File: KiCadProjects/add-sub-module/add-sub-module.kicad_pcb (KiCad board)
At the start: 2 copper layers, 56 x 68 mm, 32 parts, among them J1 2x4_Header, J2 1x2_Header, M1 MountingHole_2.2mm_M2_Pad, M2 MountingHole_2.2mm_M2_Pad, M3 MountingHole_2.2mm_M2_Pad, M4 MountingHole_2.2mm_M2_Pad

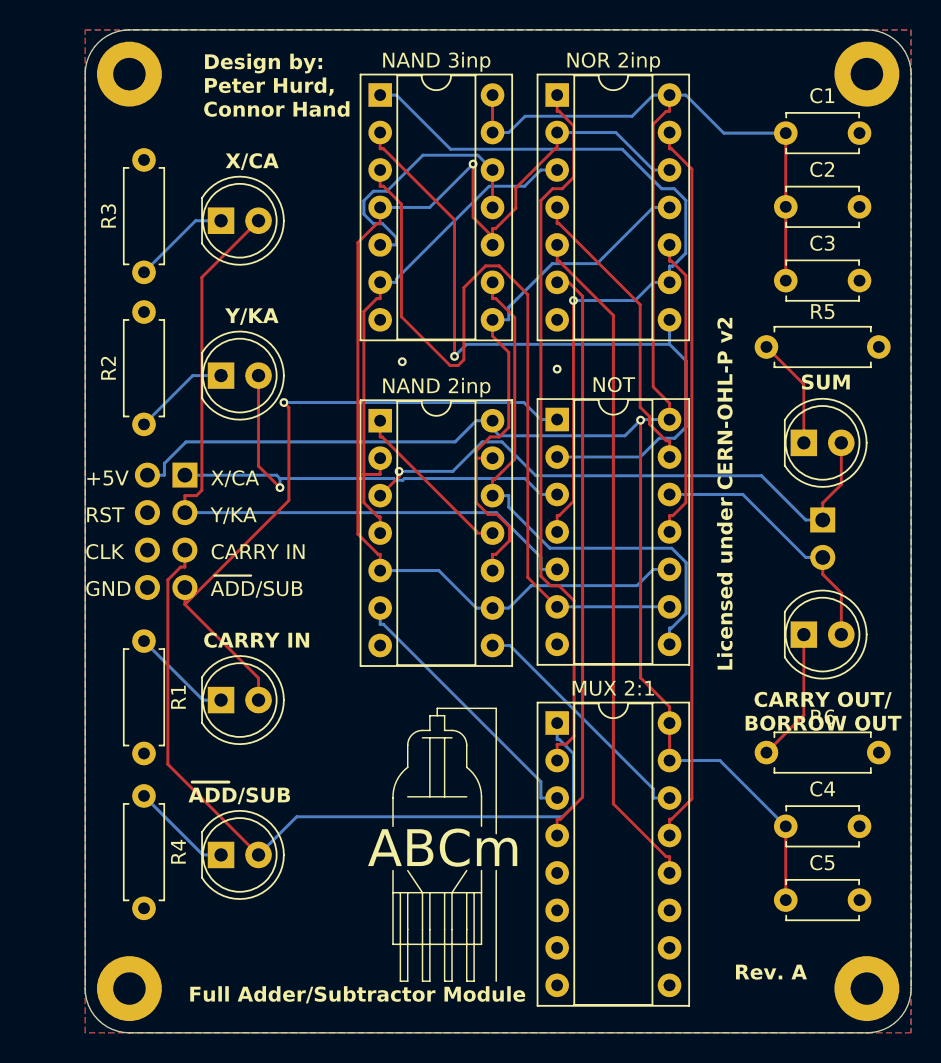
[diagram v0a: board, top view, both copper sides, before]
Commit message: final updates for Revision A
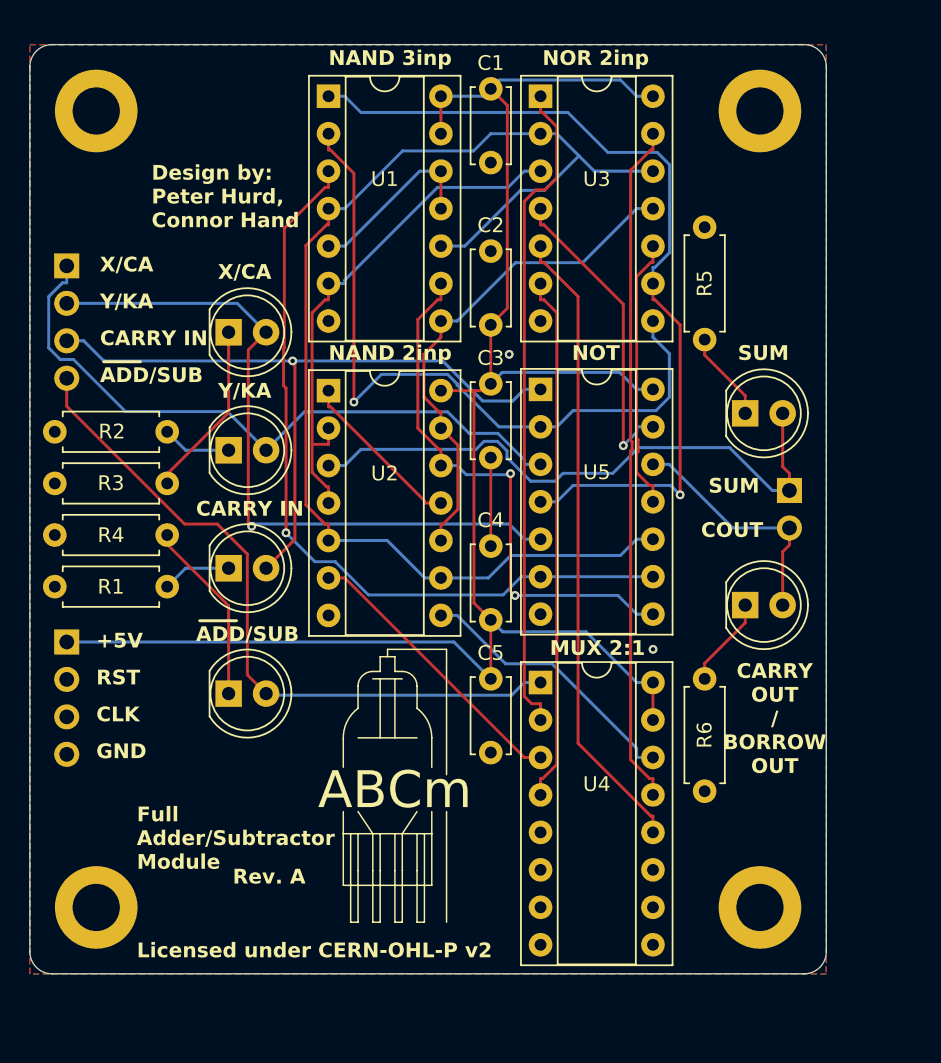
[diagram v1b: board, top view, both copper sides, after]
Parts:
- removed M1, M2, M3, M4: MountingHole_2.2mm_M2_Pad, MountingHole:MountingHole_2.2mm_M2_Pad
- added H1: MountingHole_Pad, MountingHole:MountingHole_3.2mm_M3_DIN965_Pad, F.Cu at (100.2, 67.0)
- added H2: MountingHole_Pad, MountingHole:MountingHole_3.2mm_M3_DIN965_Pad, F.Cu at (145.2, 67.0)
- added H3: MountingHole_Pad, MountingHole:MountingHole_3.2mm_M3_DIN965_Pad, F.Cu at (100.2, 121.0)
- added H4: MountingHole_Pad, MountingHole:MountingHole_3.2mm_M3_DIN965_Pad, F.Cu at (145.2, 121.0)
- added J3: Conn_01x02_Pin, Connector_PinHeader_2.54mm:PinHeader_1x02_P2.54mm_Vertical, B.Cu at (147.2, 92.7)
- C1, C2, C3, C4, C5: footprint Capacitor_THT:C_Disc_D4.7mm_W2.5mm_P5.00mm -> Capacitor_THT:C_Disc_D5.0mm_W2.5mm_P5.00mm
- J1: value 2x4_Header -> Conn_01x04_Pin; footprint Connector_PinHeader_2.54mm:PinHeader_2x04_P2.54mm_Vertical -> Connector_PinHeader_2.54mm:PinHeader_1x04_P2.54mm_Vertical
- J2: value 1x2_Header -> Conn_01x04_Pin; footprint Connector_PinHeader_2.54mm:PinHeader_1x02_P2.54mm_Vertical -> Connector_PinHeader_2.54mm:PinHeader_1x04_P2.54mm_Vertical
- R1, R2, R3, R4, R5, R6: value 1k -> 330
- U1: renamed from NAND 3inp
- U2: renamed from NAND 2inp
- U3: renamed from NOR 2inp
- U4: renamed from MUX 2:1
- moved J2 54.1 mm to (98.2, 77.5)
- moved G*** 30.6 mm to (146.0, 76.0)
- moved C5 25.0 mm to (127.0, 105.5), turned to -90 degrees
- moved C4 24.4 mm to (127.0, 101.5), turned to 90 degrees
- moved C2 21.5 mm to (127.0, 81.5), turned to 90 degrees
- moved C3 21.2 mm to (127.0, 85.5), turned to -90 degrees
- moved C1 20.2 mm to (127.0, 65.5), turned to -90 degrees
- moved R4 17.8 mm to (105.1, 95.8), turned to 180 degrees
- moved R3 14.4 mm to (105.1, 92.2), turned to 180 degrees
- moved J1 13.9 mm to (98.2, 103.0)
- moved D4 11.0 mm to (109.2, 106.5)
- moved D1 8.95 mm to (109.2, 98.0)
- moved REF** 7.60 mm to (108.5, 74.2)
- moved D3 7.58 mm to (109.2, 82.0)
- moved R6 6.52 mm to (141.5, 105.5), turned to -90 degrees
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- renumbered NOT to U5
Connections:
- J1 pad 1: KA -> +5V
- J1 pad 2: +5V -> CLK
- J1 pad 3: CA -> RST
- J1 pad 4: RST -> GND
- J2 pad 1: SUM -> KA
- J2 pad 2: COUT -> CA
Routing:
- net +5V: track 135.0 -> 119.2 mm, vias 1 -> 0
- net KA: track 34.7 -> 45.2 mm, vias 1 -> 0
- net Net-(U1-1Y): track 18.3 -> 12.3 mm
- net Net-(U1-2B): track 79.1 -> 85.2 mm, vias 1 -> 0
- net GND: track 0.00 -> 6.00 mm
- net Net-(U1-1A): track 53.1 -> 59.0 mm
- net Net-(D4-K): track 6.88 -> 12.5 mm
- net ADD/SUB: track 52.7 -> 47.3 mm
- net Net-(D3-K): track 6.67 -> 12.0 mm
- net Net-(U3-1Y): track 49.1 -> 44.9 mm
- net Net-(U3-2B): track 39.5 -> 35.8 mm
- net CARRY: track 45.5 -> 49.1 mm
- net Net-(U1-2A): track 56.7 -> 53.1 mm, vias 0 -> 1
- net Net-(D6-K): track 9.05 -> 6.14 mm
- net Net-(U1-3Y): track 37.4 -> 34.5 mm
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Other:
- board size 56 x 68 mm -> 54 x 63 mm
- board text added: "CARRY OUT / BORROW OUT"
- board text added: "COUT"
- board text added: "MUX 2:1"
- board text added: "NAND 2inp"
- board text added: "NAND 3inp"
- board text added: "NOR 2inp"
- board text added: "NOT"
- board text removed: "CARRY OUT/ BORROW OUT"

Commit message: FINAL FINAL final updates for Rev. A
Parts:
- U1: value CD74HCT10E -> IC-14P
- U2: value SN74HCT00N -> IC-14P
- U3: value SN74HCT02N -> IC-14P
- U4: value SN74HCT257N -> IC-16P
- U5: value CD74HCT04E -> IC-14P
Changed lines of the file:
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@@
 			)
 		)
-		(property "Value" "SN74HCT257N"
+		(property "Value" "IC-16P"
 			(at 3.81 20.11 0)
 			(layer "F.Fab")
@@
 			)
 		)
-		(property "Datasheet" "SN74HCT257N"
+		(property "Datasheet" ""
 			(at 0 0 0)
 			(unlocked yes)
@@
 			)
 		)
-		(property "Description" ""
+		(property "Description" "SN74HCT257N"
 			(at 0 0 0)
 			(unlocked yes)
@@
 			)
 		)
-		(property "Value" "CD74HCT10E"
+		(property "Value" "IC-14P"
 			(at 3.81 17.57 0)
 			(layer "F.Fab")
@@
 			)
 		)
-		(property "Datasheet" "CD74HCT10E"
+		(property "Datasheet" ""
 			(at 0 0 0)
 			(unlocked yes)
@@
 			)
 		)
-		(property "Description" ""
+		(property "Description" "CD74HCT10E"
 			(at 0 0 0)
 			(unlocked yes)
@@
 			)
 		)
-		(property "Value" "SN74HCT00N"
+		(property "Value" "IC-14P"
 			(at 3.81 17.57 0)
 			(layer "F.Fab")
@@
 			)
 		)
-		(property "Datasheet" "SN74HCT00N"
+		(property "Datasheet" ""
 			(at 0 0 0)
 			(unlocked yes)
@@
 			)
 		)
-		(property "Description" ""
+		(property "Description" "SN74HCT00N"
 			(at 0 0 0)
 			(unlocked yes)
@@
 			)
 		)
-		(property "Value" "SN74HCT02N"
+		(property "Value" "IC-14P"
 			(at 3.81 17.57 0)
 			(layer "F.Fab")
@@
 			)
 		)
-		(property "Datasheet" "SN74HCT02N"
+		(property "Datasheet" ""
 			(at 0 0 0)
 			(unlocked yes)
@@
 			)
 		)
-		(property "Description" ""
+		(property "Description" "SN74HCT02N"
 			(at 0 0 0)
 			(unlocked yes)
@@
 			)
 		)
-		(property "Value" "CD74HCT04E"
+		(property "Value" "IC-14P"
 			(at 3.81 17.57 0)
 			(layer "F.Fab")
@@
 			)
 		)
-		(property "Datasheet" "CD74HCT04E"
+		(property "Datasheet" ""
 			(at 0 0 0)
 			(unlocked yes)
@@
 			)
 		)
-		(property "Description" ""
+		(property "Description" "CD74HCT04E"
 			(at 0 0 0)
 			(unlocked yes)
